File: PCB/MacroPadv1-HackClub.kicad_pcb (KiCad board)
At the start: 2 copper layers, 84.5 x 137.7 mm, 33 parts, among them SW1 SW_Push, SW10 SW_Push, SW11 SW_Push, SW12 SW_Push, SW13 SW_Push, SW14 SW_Push, SW15 SW_Push, SW16 SW_Push, SW2 SW_Push, SW3 SW_Push, SW4 SW_Push, SW5 SW_Push, SW6 SW_Push, SW7 SW_Push, SW8 SW_Push, SW9 SW_Push, U1 XIAO-RP2040-DIP

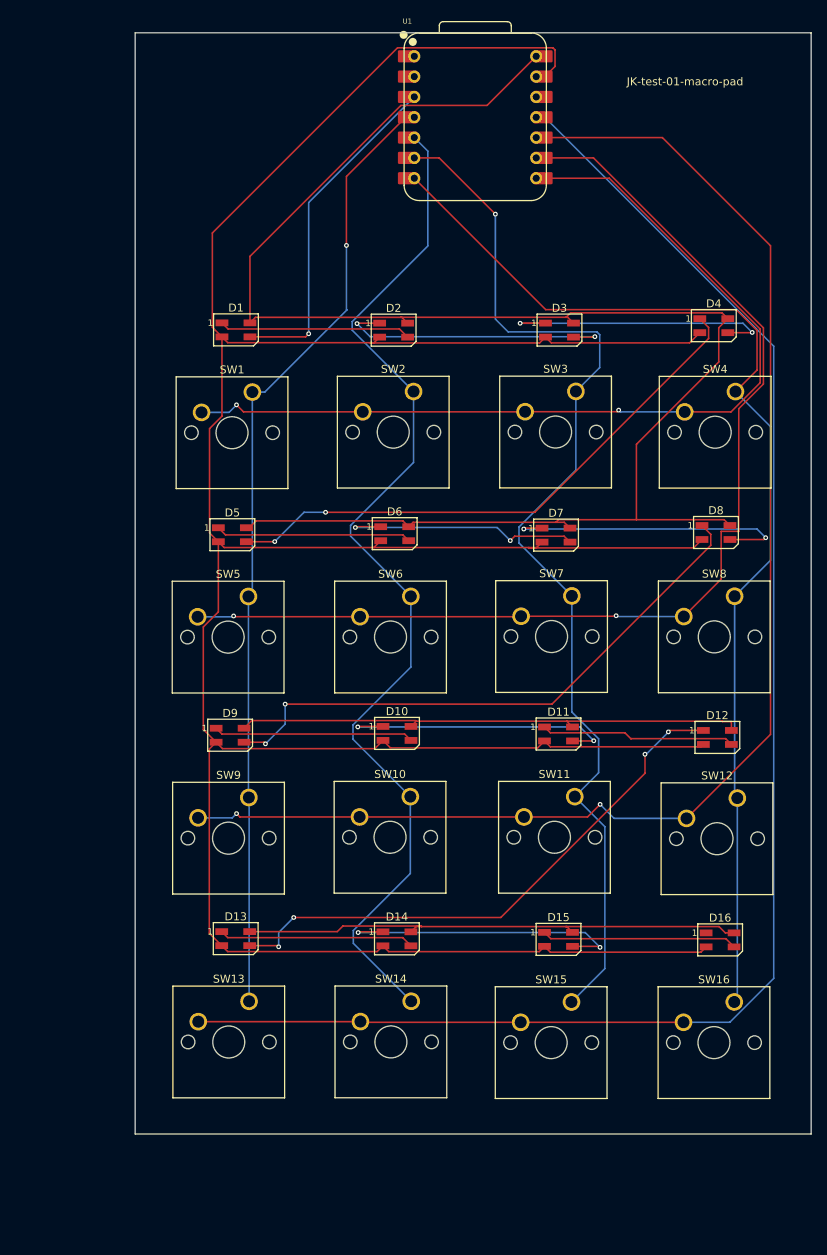
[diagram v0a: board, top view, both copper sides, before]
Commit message: Pcb rerouting
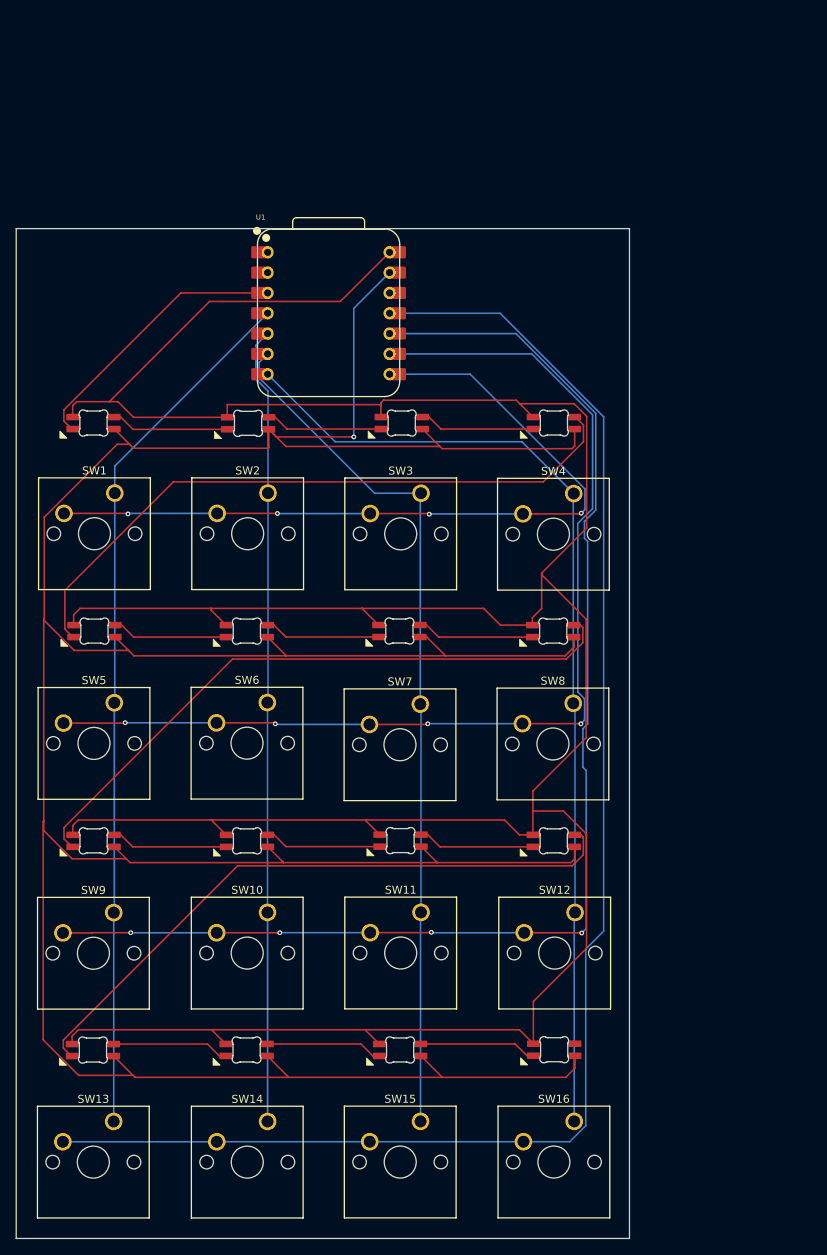
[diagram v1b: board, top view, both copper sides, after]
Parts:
- D1, D10, D11, D12, D13, D14, D15, D16, D2, D3, D4, D5, D6, D7, D8, D9: value SK6812MINI -> SK6812MINI-E; footprint LED_SMD:LED_SK6812MINI_PLCC4_3.5x3.5mm_P1.75mm -> kicad-keyboard-parts.pretty-master:MX_SK6812MINI-E; moved to B.Cu
- moved U1 30.6 mm to (129.7, 61.6)
- moved SW16 25.0 mm to (160.4, 162.6)
- moved SW12 24.8 mm to (160.5, 136.5)
- moved SW8 24.2 mm to (160.3, 110.3)
- moved SW15 24.1 mm to (141.2, 162.6)
- moved SW11 24.1 mm to (141.2, 136.5)
- moved SW4 23.9 mm to (160.3, 84.1)
- moved SW14 23.4 mm to (122.1, 162.6)
- moved SW7 23.3 mm to (141.1, 110.4)
- moved SW3 23.2 mm to (141.2, 84.1)
- moved SW10 23.0 mm to (122.0, 136.5)
- moved SW13 22.6 mm to (102.8, 162.6)
- moved D16 22.5 mm to (157.9, 148.6), turned to 180 degrees
- moved SW6 22.3 mm to (122.0, 110.2)
- moved SW2 22.2 mm to (122.1, 84.0)
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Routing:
- net +5V: track 339.9 -> 414.8 mm
- net Net-(U1-GPIO6/SDA): track 134.1 -> 99.8 mm
- net Net-(U1-GPIO7/SCL): track 136.3 -> 108.3 mm, vias 1 -> 0
- net Net-(D14-DOUT): track 37.6 -> 14.6 mm, vias 2 -> 0
- net Net-(D7-DOUT): track 37.6 -> 14.7 mm, vias 2 -> 0
- net Net-(D10-DOUT): track 36.1 -> 14.6 mm, vias 2 -> 0
- net Net-(D2-DOUT): track 36.0 -> 14.6 mm, vias 2 -> 0
- net Net-(D3-DOUT): track 35.7 -> 14.4 mm, vias 2 -> 0
- net GND: track 402.7 -> 420.2 mm, vias 0 -> 1
- net Net-(D6-DOUT): track 31.3 -> 14.5 mm, vias 2 -> 0
- net Net-(U1-GPIO0/TX): track 139.8 -> 123.1 mm
- net Net-(U1-GPIO1/RX): track 114.8 -> 98.4 mm, vias 2 -> 4
- net Net-(U1-GPIO29/ADC3/A3): track 120.7 -> 109.0 mm, vias 1 -> 0
- net Net-(U1-GPIO4/MISO): track 172.8 -> 161.2 mm, vias 2 -> 4
- net Net-(D4-DOUT): track 71.2 -> 82.5 mm, vias 2 -> 0
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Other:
- board size 84.5 x 137.7 mm -> 76.7 x 126.2 mm
- board text added: "JK-test-02-hackpad"
- board text removed: "JK-test-01-macro-pad"
